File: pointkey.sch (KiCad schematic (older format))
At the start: 18 parts, among them K1 RELAY_1RT, P1 CONN_01X02, P2 CONN_01X03, Q1 КТ315, Q2 КТ315, SW1 SW_PUSH, U1 4013

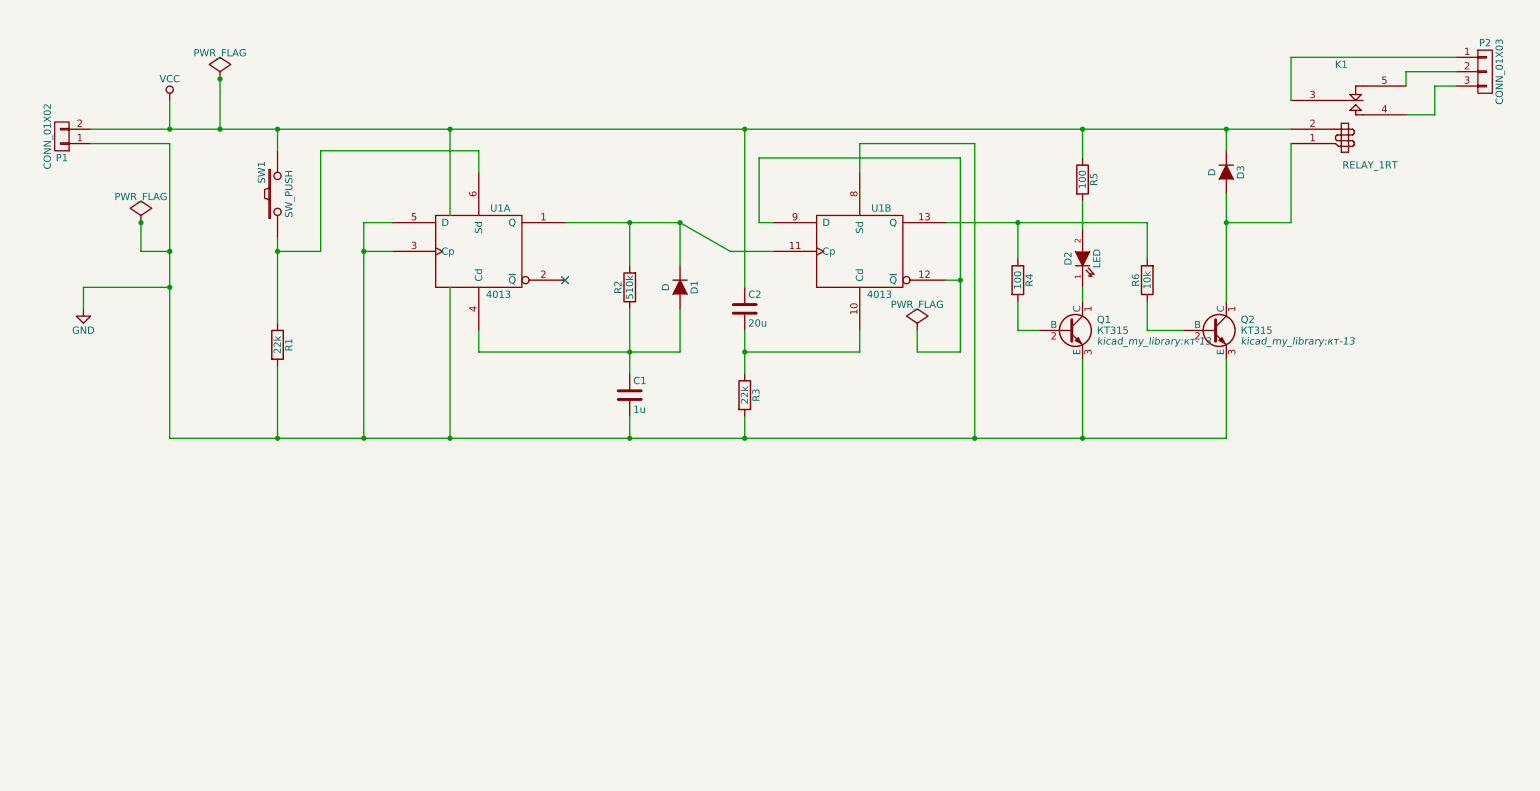
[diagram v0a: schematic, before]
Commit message: dispatcher
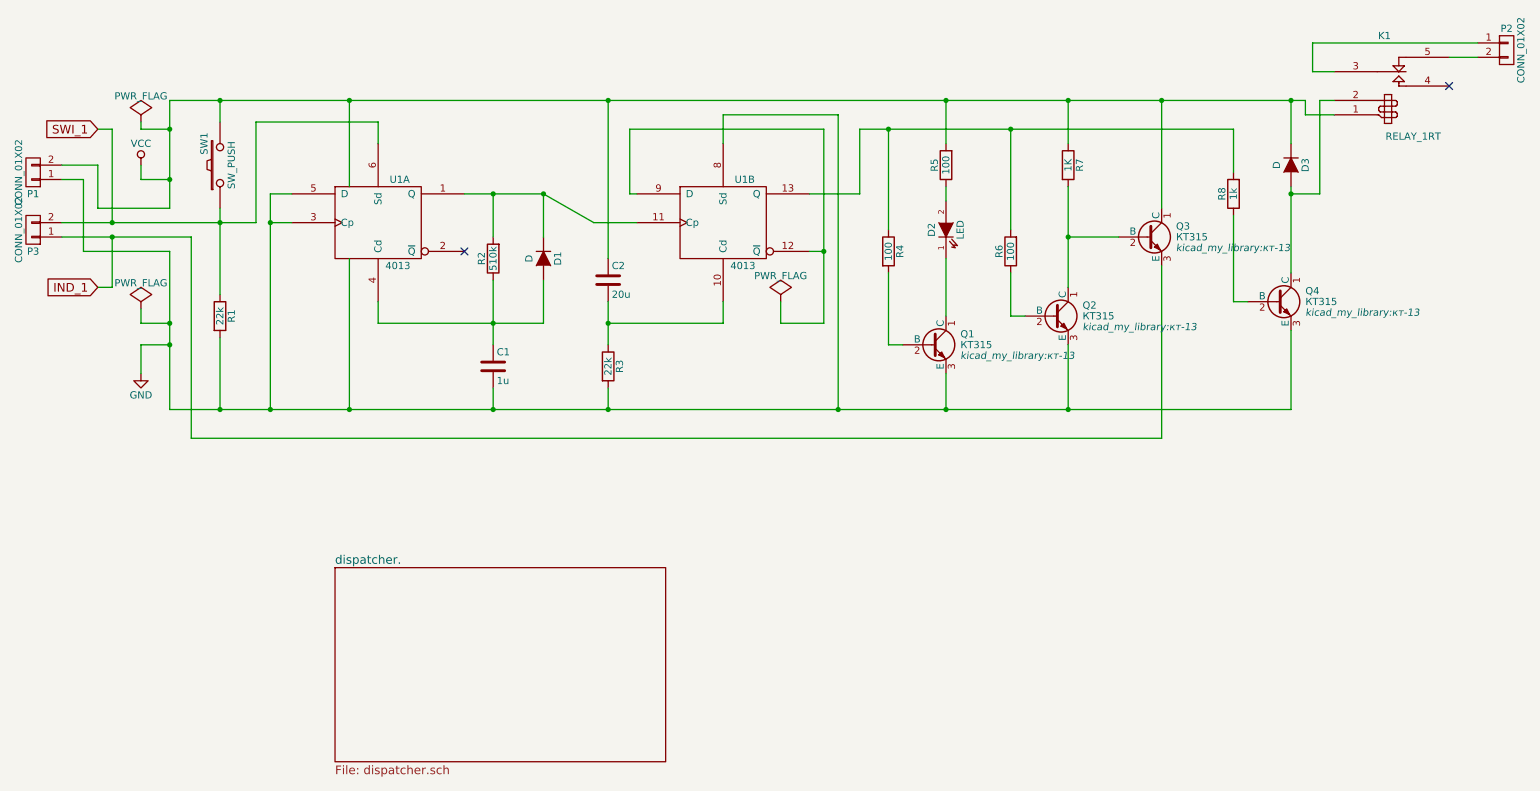
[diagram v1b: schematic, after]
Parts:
- removed P2: CONN_01X03, Pin_Headers:Pin_Header_Straight_1x03, symbol CONN_01X03
- added P2, P3: CONN_01X02, Connect:AK300-2, symbol CONN_01X02
- added Q2, Q3: КТ315, kicad_my_library:кт-13, symbol КТ315
- added R6: 100, Discret:R3-5, symbol R
- added R7: 1K, Discret:R3-5, symbol R
- P1: footprint Pin_Headers:Pin_Header_Straight_1x02 -> Connect:AK300-2
- R8: renamed from R6; value 10k -> 1k
- renumbered Q2 to Q4
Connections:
- net GND: now also Q2.3 (E)
- net VCC: now also K1.1, R5.2, Q3.1 (C), R7.1; no longer K1.2, R5.1
- net SWI_1: now reaches R1.1, SW1.1, U1.6 (Sd)
- net SWI_1: now also P3.2 (P2)
- net at R4.1, R8.2, U1.13 (Q): now also R6.2
- net at D3.2 (A), Q4.1 (C): now also K1.2; no longer K1.1
- net at K1.3: now also P2.1 (P1)
- net at K1.5: now also P2.2 (P2)
- net at D2.2 (A): now also R5.1; no longer R5.2
- new net: Q2.2 (B), R6.1
- new net: Q2.1 (C), Q3.2 (B), R7.2
- new net IND_1: P3.1 (P1), Q3.3 (E)
- no-connect marks 1 -> 2
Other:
- moved on the sheet: C1, C2, D1, D2, D3, K1, Q1, Q4, R1, R2, R3, R4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
